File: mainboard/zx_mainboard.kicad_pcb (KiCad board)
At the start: 2 copper layers, 149.9 x 130.2 mm, 93 parts, among them P1 CONN_02X17, P2 CONN_02X20, P3 CONN_02X20, P4 CONN_01X02, Q1 BSS123, Q2 BSS123, Q3 BSS123, Q4 BSS123, Q5 BSS123, Q6 BSS123, Q7 BSS123, Q8 BSS123, U1 4066, U2 4066, U3 4066, U4 4066, U5 4066, U6 74HC14, U7 74HC14

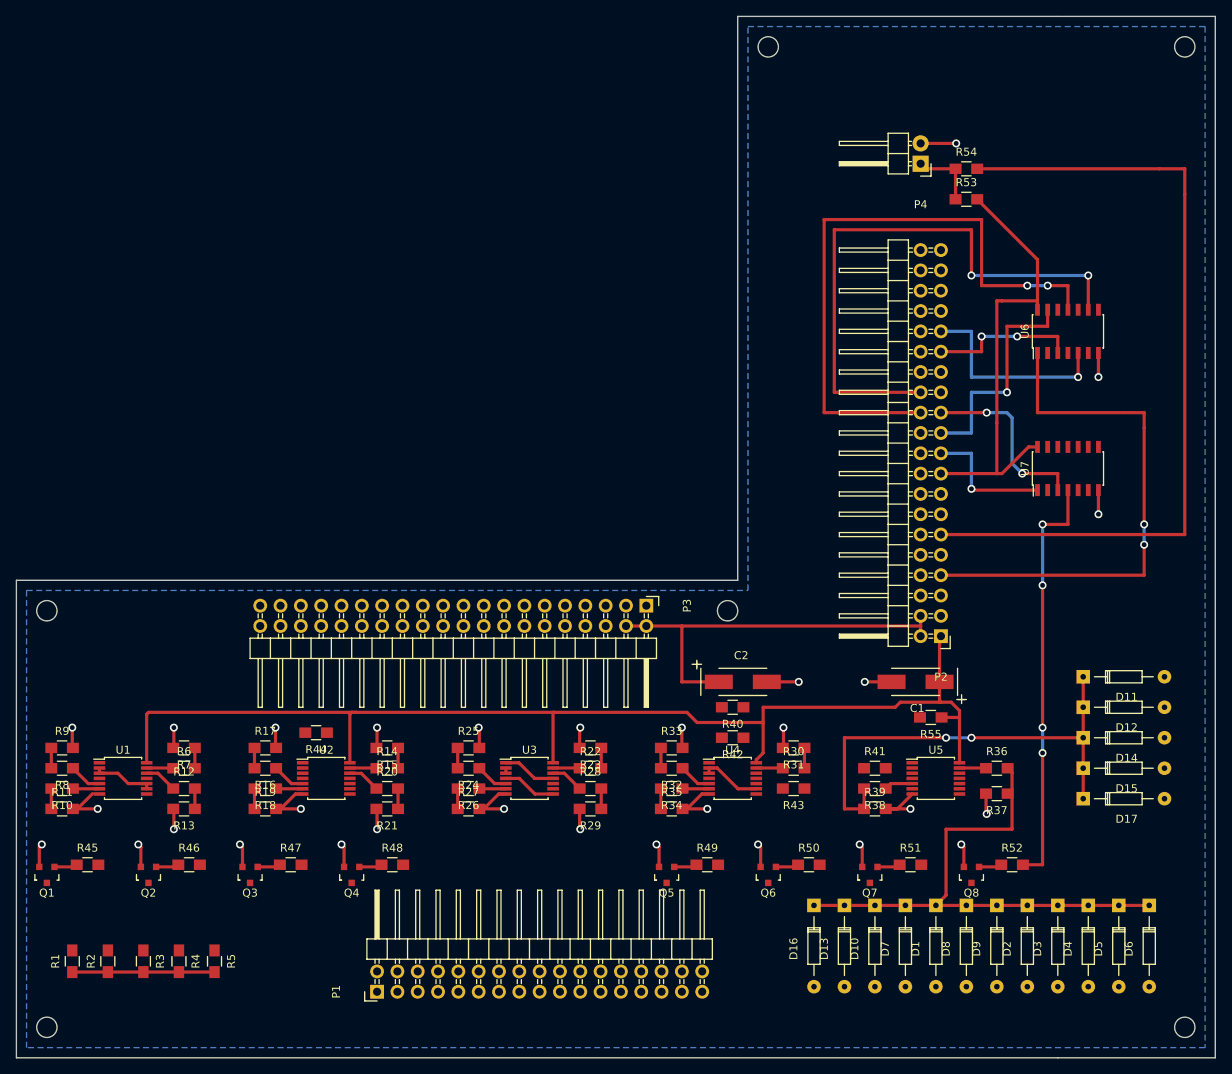
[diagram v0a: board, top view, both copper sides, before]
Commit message: pcb
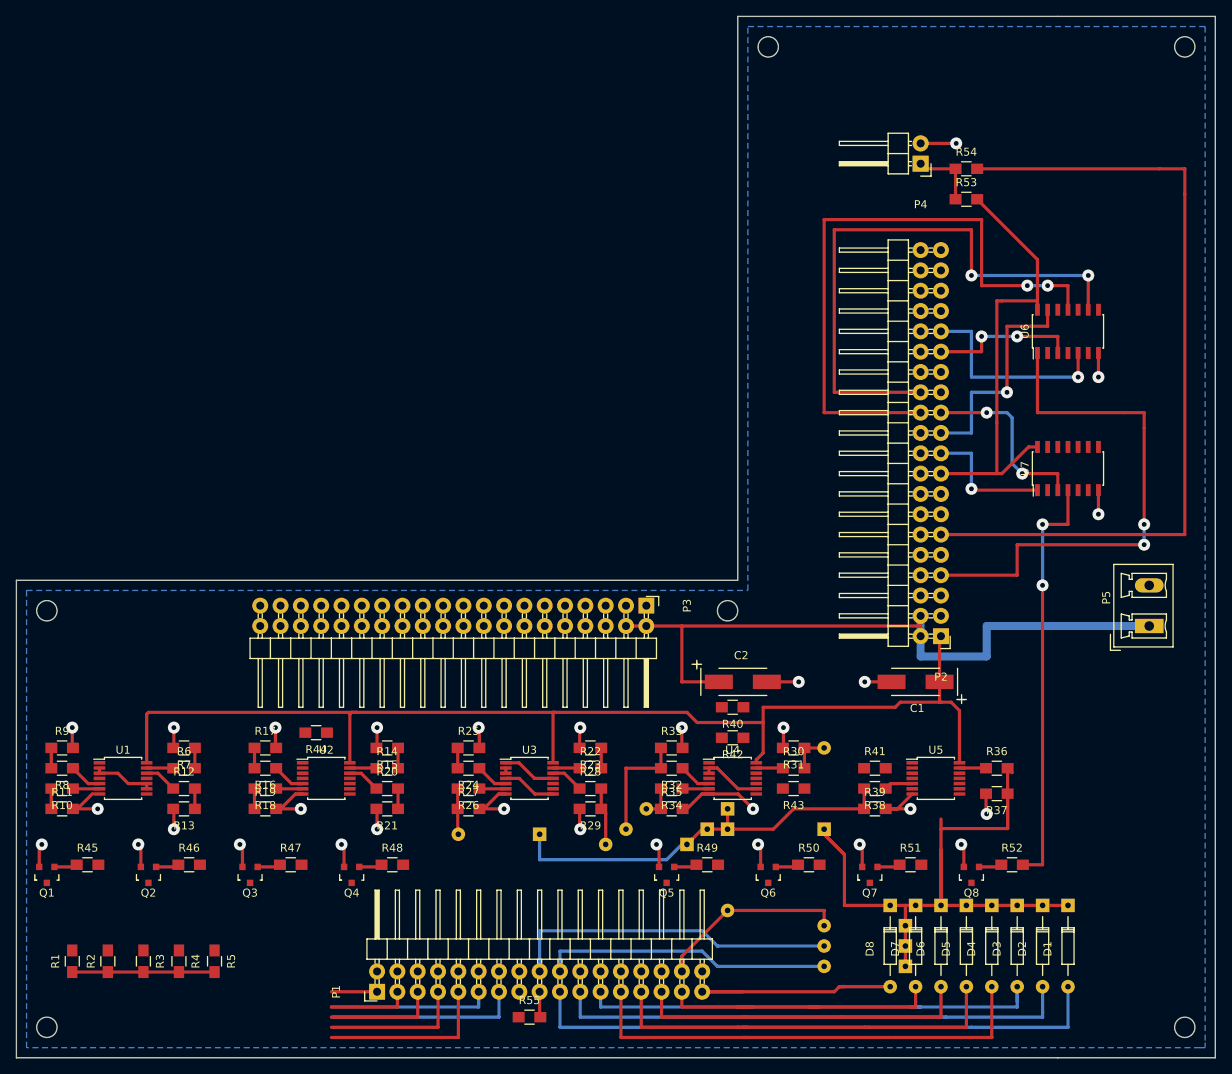
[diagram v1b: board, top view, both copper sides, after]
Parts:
- added P5: CONN_01X02, Connectors_Phoenix:PhoenixContact_MCV-G_02x5.08mm_Vertical, F.Cu at (184.2, 92.7)
- D10, D11, D12, D13, D14, D15, D16, D17, D9: moved to B.Cu
- moved D11 70.7 mm to (108.0, 118.7), turned to 180 degrees
- moved R55 62.6 mm to (106.7, 141.6), turned to 0 degrees
- moved D12 52.4 mm to (126.4, 120.0), turned to 180 degrees
- moved D14 48.4 mm to (128.9, 118.1), turned to 180 degrees
- moved D15 44.7 mm to (131.4, 115.6), turned to 180 degrees
- moved D17 44.6 mm to (131.4, 118.1), turned to 270 degrees
- moved D6 26.0 mm to (158.1, 127.6)
- moved D5 19.0 mm to (161.3, 127.6)
- moved D1 16.5 mm to (174.0, 127.6)
- moved D9 12.5 mm to (153.7, 132.7), turned to 180 degrees
- moved D4 12.1 mm to (164.5, 127.6)
- moved D16 11.7 mm to (153.7, 130.2), turned to 180 degrees
- moved D13 9.86 mm to (143.5, 118.1), turned to 90 degrees
- moved D8 9.52 mm to (151.8, 127.6)
- moved D10 8.52 mm to (153.7, 135.3), turned to 180 degrees
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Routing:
- net /KEDIT: track 2.54 -> 76.2 mm
- net /KCL: track 2.54 -> 68.6 mm
- net /KTV: track 2.54 -> 63.5 mm
- net /KIV: track 2.54 -> 61.6 mm
- net /KLEFT: track 2.54 -> 54.6 mm
- net /KDOWN: track 2.54 -> 45.7 mm
- net +5V: track 51.0 -> 93.5 mm
- net /KGR: track 2.66 -> 44.1 mm
- net /KDEL: track 2.54 -> 38.9 mm
- net /KUP: track 2.54 -> 38.7 mm
- net /KRIGHT: track 2.54 -> 32.0 mm
- net /KD4: track 0.00 -> 24.1 mm
- net /KEXT: track 0.00 -> 24.0 mm
- net /KD0: track 6.71 -> 28.3 mm
- net /CS_CTRL: track 68.1 -> 88.6 mm
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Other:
- net class Default: via_dia 1 -> 1.5
- net class power added: clearance 0.4, trace_width 1, via_dia 1.5, via_drill 0.6
